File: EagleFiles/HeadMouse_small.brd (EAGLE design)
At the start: 86 x 45.7 mm, 12 parts

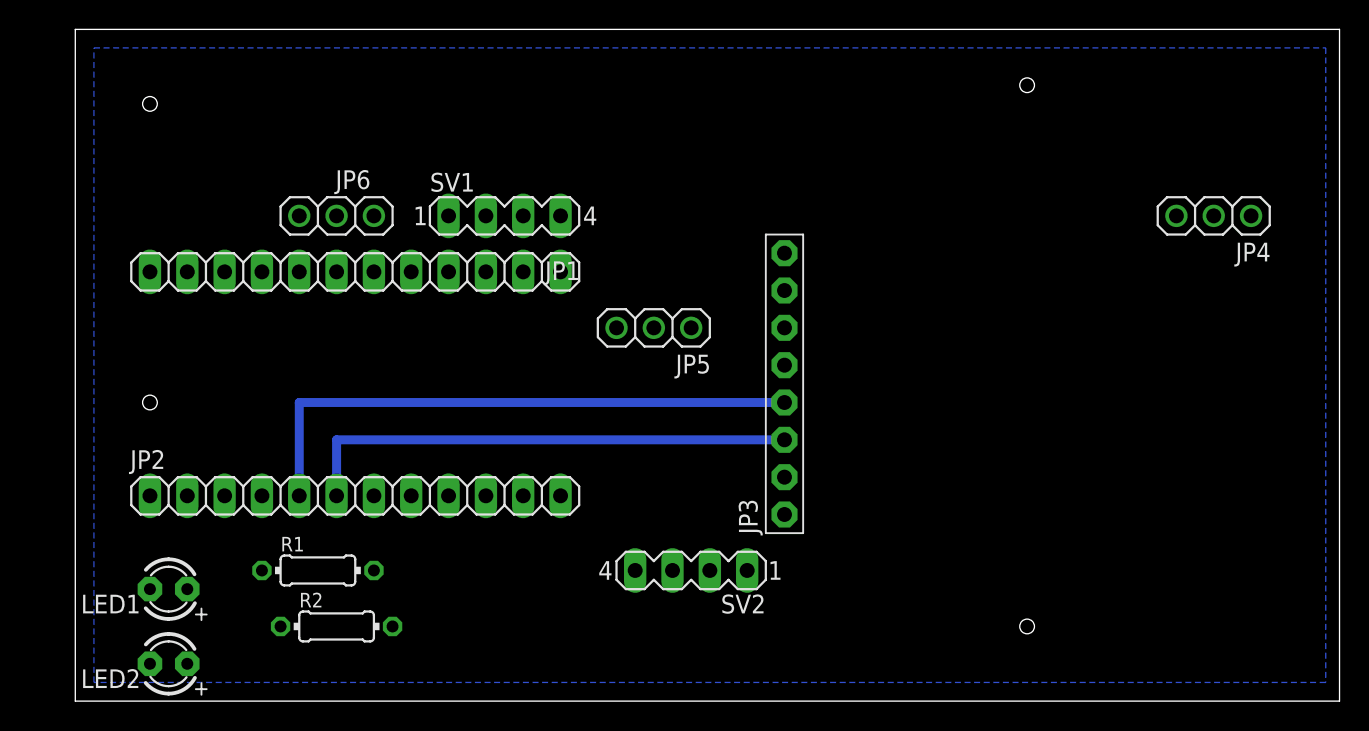
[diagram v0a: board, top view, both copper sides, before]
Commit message: Fixed mistake in the Eagle folder
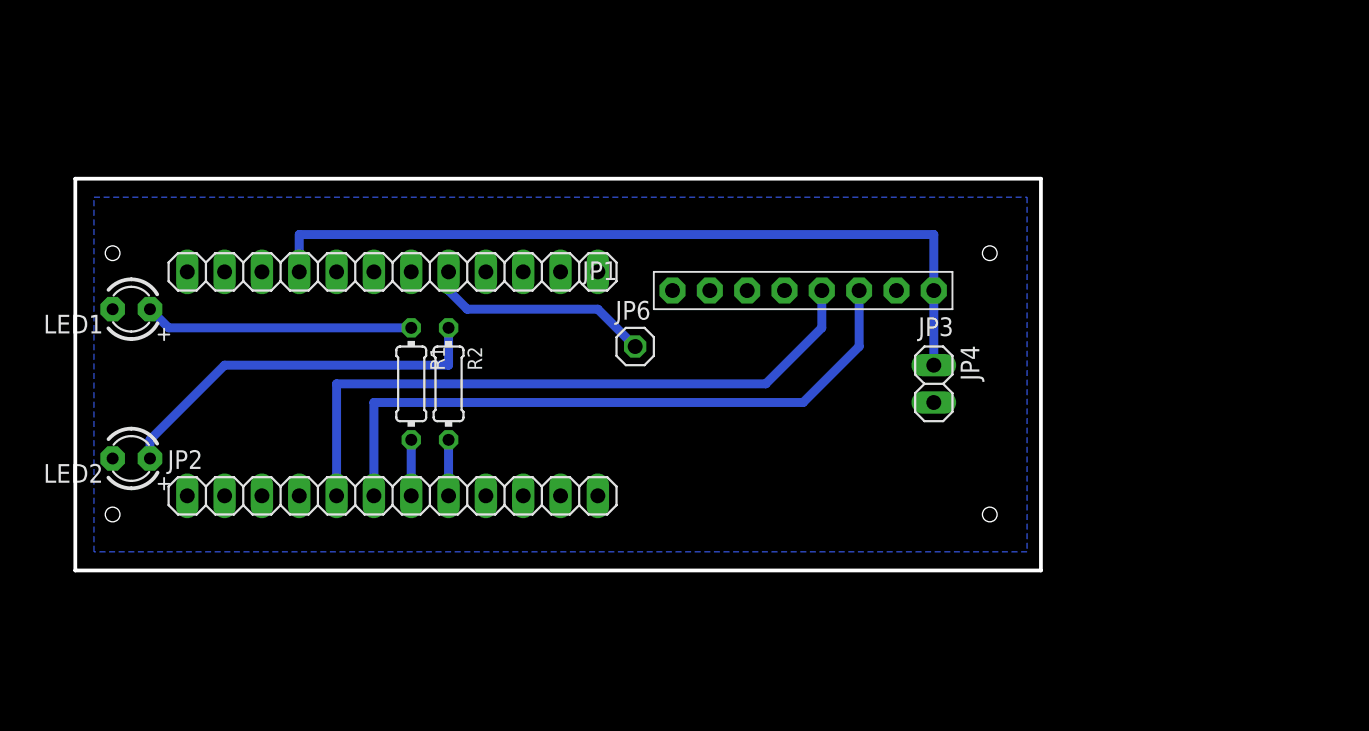
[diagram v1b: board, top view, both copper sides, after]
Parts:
- removed JP5: (no value), adafruit:1X03
- removed SV1, SV2: (no value), con-lstb:MA04-1
- JP4: device adafruit:1X03 -> pinhead:1X02
- JP6: device adafruit:1X03 -> pinhead:1X01
- moved JP4 22.2 mm to (58.4, 21.6), turned to 270 degrees
- moved JP6 22.2 mm to (38.1, 24.1)
- moved LED1 19.2 mm to (3.81, 26.7)
- moved R2 18.2 mm to (25.4, 21.6), turned to 270 degrees
- moved LED2 14.2 mm to (3.81, 16.5)
- moved R1 14.2 mm to (22.9, 21.6), turned to 270 degrees
- moved JP3 6.48 mm to (49.5, 27.9), turned to 180 degrees
- moved JP1 2.54 mm to (21.6, 29.2)
- moved JP2 2.54 mm to (21.6, 14.0)
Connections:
- removed net N$10: JP1.4, SV1.1
- removed net N$11: JP1.3, SV1.2
- removed net N$12: JP1.2, SV1.3
- removed net N$13: JP1.1, SV1.4
- removed net N$14: JP2.9, SV2.4
- removed net N$15: JP2.10, SV2.3
- removed net N$16: JP2.11, SV2.2
- removed net N$17: JP2.12, SV2.1
- net +5V: now also JP4.1; no longer JP4.2
- net GND: now also JP4.2; no longer JP4.3
- net N$7: no longer JP6.1
- net N$8: no longer JP6.2
- net N$9: no longer JP6.3
- net PRES: now also JP6.1; no longer JP5.2
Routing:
- net +5V: track 0.00 -> 54.6 mm
- net N$4: track 0.00 -> 26.2 mm
- net N$3: track 0.00 -> 18.3 mm
- net PRES: track 0.00 -> 15.5 mm
- net N$6: track 34.3 -> 44.8 mm
- net N$1: track 39.4 -> 44.8 mm
- net N$5: track 0.00 -> 3.81 mm
- net N$2: track 0.00 -> 3.81 mm
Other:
- board size 86 x 45.7 mm -> 65.7 x 26.7 mm
